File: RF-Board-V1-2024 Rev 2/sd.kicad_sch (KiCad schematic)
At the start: 8 parts, among them J9 MSD-10-C

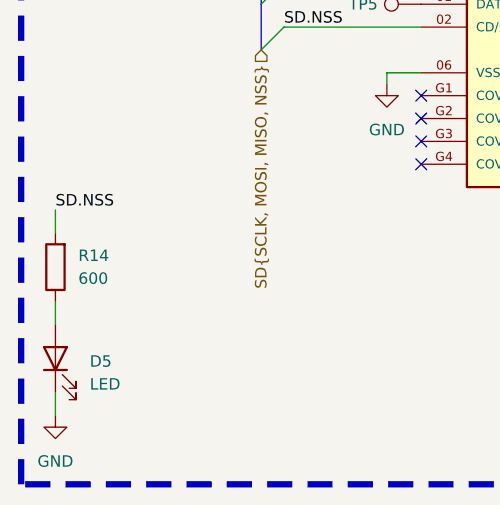
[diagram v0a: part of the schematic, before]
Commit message: made some notes
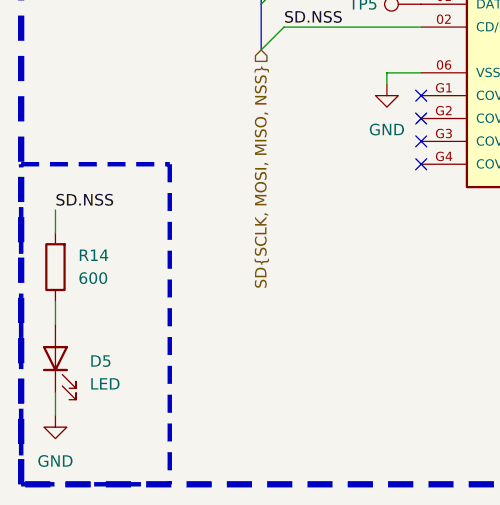
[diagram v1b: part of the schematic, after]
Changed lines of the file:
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@@
 (kicad_sch
-	(version 20231120)
+	(version 20250114)
 	(generator "eeschema")
-	(generator_version "8.0")
+	(generator_version "9.0")
 	(paper "A4")
 	(title_block
@@
 		(company "University Of Alberta EcoCar Team")
 	)
+	(rectangle
+		(start 13.97 81.28)
+		(end 30.48 116.84)
+		(stroke
+			(width 0.5)
+			(type dash)
+			(color 255 0 0 1)
+		)
+		(fill
+			(type none)
+		)
+	)
+	(rectangle
+		(start 13.97 17.78)
+		(end 88.9 116.84)
+		(stroke
+			(width 0.7)
+			(type dash)
+		)
+		(fill
+			(type none)
+		)
+	)
+	(text "MSD-10-C (microSD)"
+		(exclude_from_sim no)
+		(at 13.97 16.256 0)
+		(effects
+			(font
+				(size 2 2)
+				(thickness 0.4)
+				(bold yes)
+				(italic yes)
+			)
+			(justify left bottom)
+		)
+	)
 	(junction
 		(at 58.42 27.94)
@@
 		)
 	)
-	(rectangle
-		(start 13.97 17.78)
-		(end 88.9 116.84)
-		(stroke
-			(width 0.7)
-			(type dash)
-		)
-		(fill
-			(type none)
-		)
-	)
-	(text "MSD-10-C (microSD)"
-		(exclude_from_sim no)
-		(at 13.97 16.256 0)
-		(effects
-			(font
-				(size 2 2)
-				(thickness 0.4)
-				(bold yes)
-				(italic yes)
-			)
-			(justify left bottom)
-		)
-	)
 	(label "SD.NSS"
 		(at 17.78 86.36 0)
-		(fields_autoplaced yes)
 		(effects
 			(font
@@
 	(label "SD.NSS"
 		(at 43.18 66.04 0)
-		(fields_autoplaced yes)
 		(effects
 			(font
@@
 	(label "SD.MOSI"
 		(at 43.18 53.34 0)
-		(fields_autoplaced yes)
 		(effects
 			(font
@@
 	(label "SD.SCLK"
 		(at 43.18 48.26 0)
-		(fields_autoplaced yes)
 		(effects
 			(font
@@
 	(label "SD.MISO"
 		(at 43.18 60.96 0)
-		(fields_autoplaced yes)
 		(effects
 			(font
@@
 		(shape input)
 		(at 40.64 68.58 270)
-		(fields_autoplaced yes)
-		(effects
-			(font
+		(effects
+			(font
